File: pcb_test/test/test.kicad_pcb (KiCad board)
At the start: 2 copper layers, 14 parts, among them T2 BC817, T3 BC847BPN

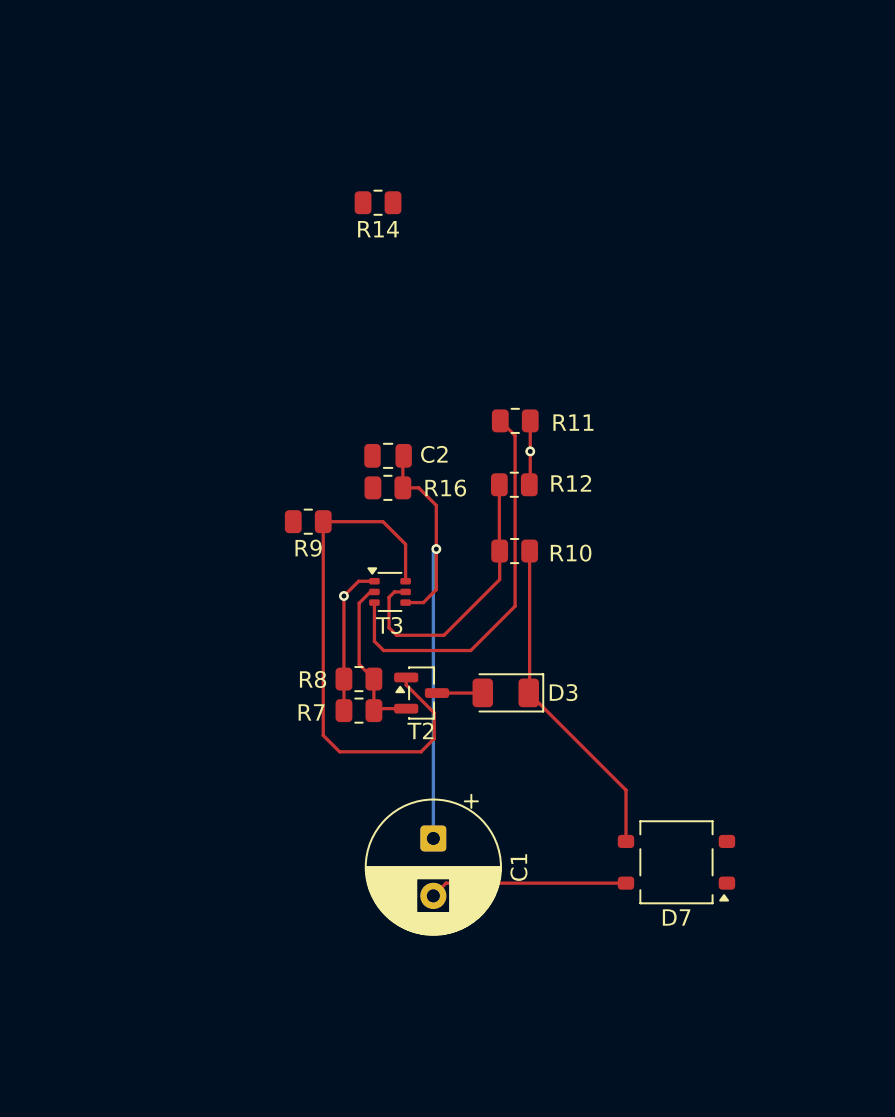
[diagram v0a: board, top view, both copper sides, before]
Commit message: WIP
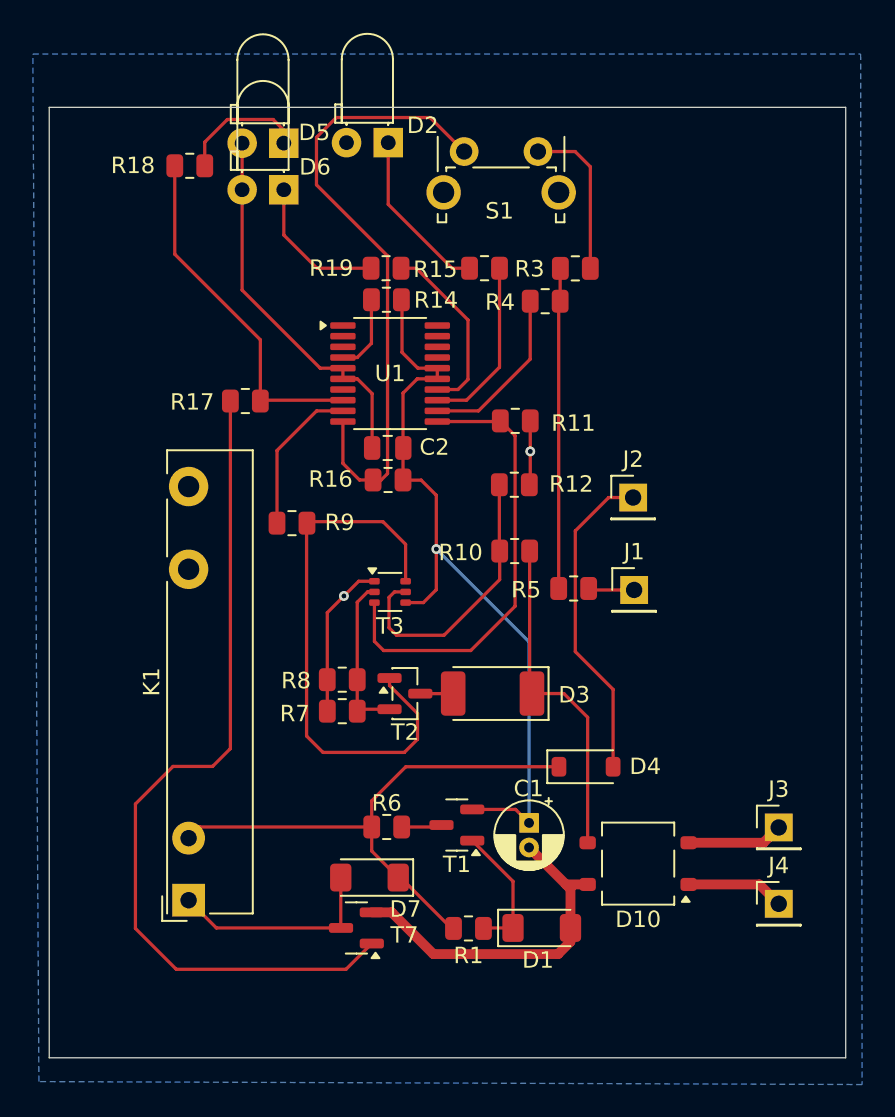
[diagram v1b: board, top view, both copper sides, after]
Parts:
- added D1: 5V6, Diode_SMD:D_MiniMELF, F.Cu at (98.3, 122.5)
- added D2: LED, LED_THT:LED_D3.0mm_Horizontal_O1.27mm_Z2.0mm, F.Cu at (89.0, 74.6)
- added D4: 1N4148W, Diode_SMD:D_SOD-123, F.Cu at (101.0, 112.7)
- added D5: LED, LED_THT:LED_D3.0mm_Horizontal_O1.27mm_Z2.0mm, F.Cu at (82.6, 77.5)
- added D6: LED, LED_THT:LED_D3.0mm_Horizontal_O1.27mm_Z2.0mm, F.Cu at (82.6, 74.7)
- added D7: LL4148, Diode_SMD:D_MiniMELF, F.Cu at (87.8, 119.4)
- added J1: M- Eingang, Connector_PinHeader_2.54mm:PinHeader_1x01_P2.54mm_Vertical, F.Cu at (103.9, 101.9)
- added J2: P Eingang 24V, Connector_PinHeader_2.54mm:PinHeader_1x01_P2.54mm_Vertical, F.Cu at (103.9, 96.3)
- added J3: BUS IN, Connector_PinHeader_2.54mm:PinHeader_1x01_P2.54mm_Vertical, F.Cu at (112.8, 116.4)
- added J4: BUS IN, Connector_PinHeader_2.54mm:PinHeader_1x01_P2.54mm_Vertical, F.Cu at (112.8, 121.0)
- added K1: Fujitsu_FTR-LYAA005x, Relay_THT:Relay_SPST-NO_Fujitsu_FTR-LYAA005x_FormA_Vertical, F.Cu at (76.8, 120.8)
- added R1: 47K, Resistor_SMD:R_0805_2012Metric, F.Cu at (93.8, 122.5)
- added R15: 680, Resistor_SMD:R_0805_2012Metric, F.Cu at (94.8, 82.3)
- added R17: 470, Resistor_SMD:R_0805_2012Metric, F.Cu at (80.3, 90.4)
- added R18: 680, Resistor_SMD:R_0805_2012Metric, F.Cu at (76.9, 76.0)
- added R19: 680, Resistor_SMD:R_0805_2012Metric, F.Cu at (88.8, 82.3)
- added R3: 2K2, Resistor_SMD:R_0805_2012Metric, F.Cu at (100.4, 82.3)
- added R4: 100K, Resistor_SMD:R_0805_2012Metric, F.Cu at (98.5, 84.3)
- added R5: 6K8, Resistor_SMD:R_0805_2012Metric, F.Cu at (100.3, 101.8)
- added R6: 470, Resistor_SMD:R_0805_2012Metric, F.Cu at (88.9, 116.3)
- added S1: SW_Push, Button_Switch_THT:SW_Tactile_SPST_Angled_PTS645Vx31-2LFS, F.Cu at (93.6, 75.2)
- added T1: BC817, Package_TO_SOT_SMD:SOT-23, F.Cu at (93.1, 116.2)
- added T7: BC817, Package_TO_SOT_SMD:SOT-23, F.Cu at (87.0, 122.5)
- added U1: PIC16F627A-ISS, Package_SO:SSOP-20_4.4x6.5mm_P0.65mm, F.Cu at (89.1, 88.7)
- C1: value TBD -> 47uF; footprint Capacitor_THT:CP_Radial_D8.0mm_P3.50mm -> Capacitor_THT:CP_Radial_D4.0mm_P1.50mm
- C2: value TBD -> 100nF
- D3: footprint Diode_SMD:D_1206_3216Metric -> Diode_SMD:D_MELF
- moved R14 5.93 mm to (88.8, 84.2)
- moved C1 5.91 mm to (97.5, 116.1)
- moved D10 2.34 mm to (104.2, 118.6)
- moved R7 1.02 mm to (86.2, 109.3)
- moved R8 1.02 mm to (86.2, 107.4)
- moved T2 1.02 mm to (90.0, 108.2)
- moved R9 1.00 mm to (83.1, 97.8)
- moved D3 0.80 mm to (95.3, 108.2)
- moved C2 0.48 mm to (88.9, 93.2)
- moved R16 0.48 mm to (89.0, 95.2), turned to 0 degrees
- renumbered D7 to D10
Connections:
- net MCU PIN UNTEN RECHTS renamed RB4
- C1 pad 1: Net-(T3B-E2) -> VDD
- C2 pad 1: Net-(T3B-E2) -> VDD
- C2 pad 2: MCU PIN MITTE RECHTS -> GND
- D10 pad 1: BUS_WIRE1 -> Net-(J4-Pin_1)
- D10 pad 2: BUS_WIRE2 -> Net-(J3-Pin_1)
- R14 pad 1: MCU PIN MITTE RECHTS -> VDD
- R14 pad 2: MCU PIN 4 LINKS -> Net-(U1-~{MCLR}/Vpp/RA5)
- R16 pad 1: Net-(T3B-E2) -> RB3
- R16 pad 2: MCU PIN UNTEN LINKS -> VDD
- R9 pad 2: MCU 2 PIN UNTEN LINKS -> RB2
- T3 pad 4: Net-(T3B-E2) -> VDD
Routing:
- net Net-(T7-B): track 0.00 -> 52.0 mm
- net VDD: track 0.00 -> 47.4 mm, vias 0 -> 1
- net GND: track 25.2 -> 68.1 mm
- net RB3: track 0.00 -> 38.5 mm
- net Net-(D4-K): track 0.00 -> 34.6 mm
- net Net-(T3B-E2): track 29.5 -> 0.00 mm, vias 1 -> 0
- net RB1: track 0.00 -> 21.5 mm
- net Net-(D4-A): track 0.00 -> 19.7 mm
- net Net-(R3-Pad2): track 0.00 -> 19.5 mm
- net Net-(D7-A): track 0.00 -> 13.1 mm
- net RB7: track 0.00 -> 11.1 mm
- net RB6: track 0.00 -> 10.7 mm
- net RB5: track 0.00 -> 10.5 mm
- net Net-(D2-K): track 0.00 -> 10.3 mm
- net RB2: track 0.00 -> 9.44 mm
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- added copper zone on B.Cu, net GND
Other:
- board outline added: 48.5 x 57.9 mm
